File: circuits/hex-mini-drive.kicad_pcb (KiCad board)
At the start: 2 copper layers, 19 parts

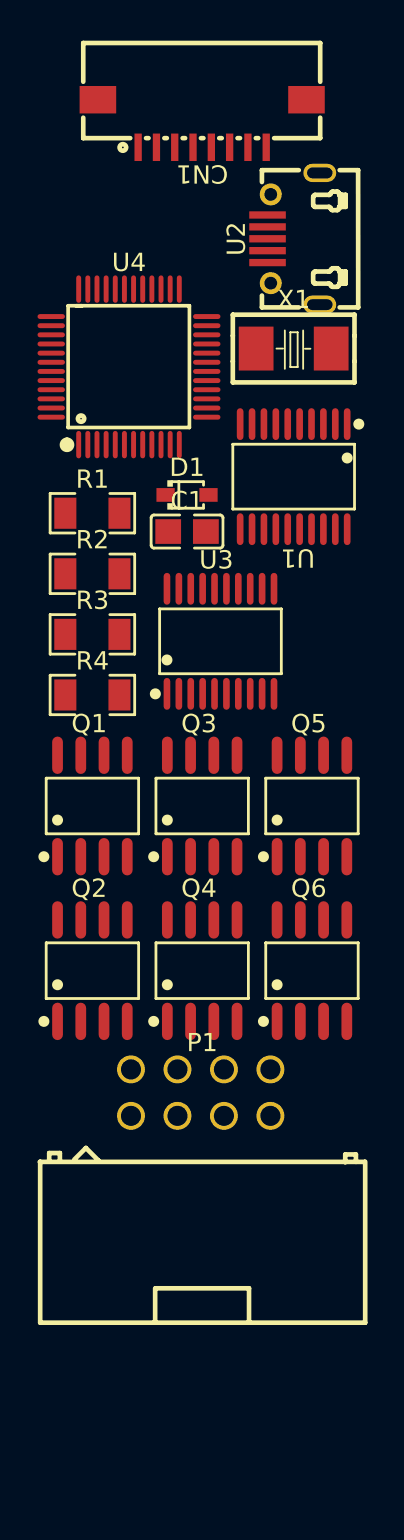
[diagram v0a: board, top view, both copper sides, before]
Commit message: Tentatively complete the PCB layout.
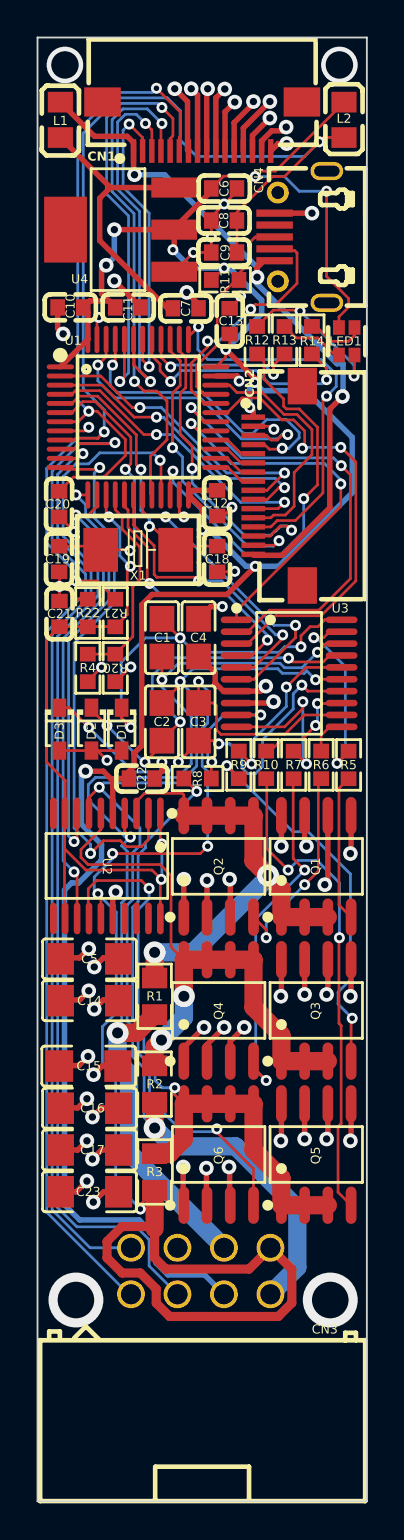
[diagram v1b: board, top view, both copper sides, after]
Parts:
- added C10: 100nF, components_footprints:C0603, F.Cu at (51.8, 64.8)
- added C11: 100nF, components_footprints:C0603, F.Cu at (55.0, 64.8)
- added C12: 100nF, components_footprints:C0603, F.Cu at (59.8, 75.5)
- added C13: 100nF, components_footprints:C0603, F.Cu at (60.5, 65.5)
- added C14: 10uF, components_footprints:C1206, F.Cu at (52.8, 102.6)
- added C15: 10uF, components_footprints:C1206, F.Cu at (52.8, 106.2)
- added C16: 10uF, components_footprints:C1206, F.Cu at (52.8, 108.5)
- added C17: 10uF, components_footprints:C1206, F.Cu at (52.8, 110.8)
- added C18: 30pF, components_footprints:C0603, F.Cu at (59.8, 78.5)
- added C19: 30pF, components_footprints:C0603, F.Cu at (51.2, 78.5)
- added C2: 10nF, components_footprints:C0805, F.Cu at (56.8, 87.4)
- added C20: 100nF, components_footprints:C0603, F.Cu at (51.2, 75.5)
- added C21: 100nF, components_footprints:C0603, F.Cu at (51.2, 81.5)
- added C22: 100nF, components_footprints:C0603, F.Cu at (55.7, 90.5)
- added C23: 10uF, components_footprints:C1206, F.Cu at (52.8, 113.1)
- added C3: 10nF, components_footprints:C0805, F.Cu at (58.8, 87.4)
- added C4: 0.1uF, components_footprints:C0805, F.Cu at (58.8, 82.8)
- added C5: 10uF, components_footprints:C1206, F.Cu at (52.8, 100.4)
- added C6: 1uF, components_footprints:C0603, F.Cu at (60.2, 58.2)
- added C7: 1uF, components_footprints:C0603, F.Cu at (58.1, 64.8)
- added C8: 100nF, components_footprints:C0603, F.Cu at (60.2, 60.0)
- added C9: 1uF, components_footprints:C0603, F.Cu at (60.2, 61.8)
- added CN2: ~, components_footprints:FPC-SMD_P0.50-16P_FGS-XJ-H2.0, F.Cu at (63.1, 74.5)
- added D2: ~, components_footprints:IN4148WS T4 SOD-323_L1.8-W1.3-LS2.5-RD, F.Cu at (53.0, 87.8)
- added D3: ~, components_footprints:IN4148WS T4 SOD-323_L1.8-W1.3-LS2.5-RD, F.Cu at (51.2, 87.8)
- added L1: 300mΩ, components_footprints:L0805, F.Cu at (51.2, 54.5)
- added L2: 10uH, components_footprints:L0805, F.Cu at (66.8, 54.5)
- added LED1: ~, components_footprints:LED-ARRAY-SMD_4P-L1.6-W1.5-BR_XL-1615RGBC-RF, F.Cu at (66.9, 66.6)
- added R10: 10Ω, components_footprints:R0603, F.Cu at (62.5, 89.8)
- added R11: 1.5kΩ, components_footprints:R0603, F.Cu at (60.3, 63.2)
- added R12: 1.5kΩ, components_footprints:R0603, F.Cu at (62.0, 66.5)
- added R13: 1.5kΩ, components_footprints:R0603, F.Cu at (63.5, 66.5)
- added R14: 1.5kΩ, components_footprints:R0603, F.Cu at (65.0, 66.5)
- added R20: 10kΩ, components_footprints:R0603, F.Cu at (54.2, 84.5)
- added R21: 47kΩ, components_footprints:R0603, F.Cu at (54.2, 81.5)
- added R22: 47kΩ, components_footprints:R0603, F.Cu at (52.8, 81.5)
- added R5: 10Ω, components_footprints:R0603, F.Cu at (67.0, 89.8)
- added R6: 10Ω, components_footprints:R0603, F.Cu at (65.5, 89.8)
- added R7: 10Ω, components_footprints:R0603, F.Cu at (64.0, 89.8)
- added R8: 10Ω, components_footprints:R0603, F.Cu at (58.7, 90.5)
- added R9: 10Ω, components_footprints:R0603, F.Cu at (61.0, 89.8)
- added U4: ~, components_footprints:AMS1117-3.3 SOT-223-3_L6.5-W3.4-P2.30-LS7.0-BR, F.Cu at (54.5, 60.5)
- C1: value ~ -> 10nF
- CN1: footprint components_footprints:FPC-SMD_KH-FG1.0-H2.0-8PIN -> components_footprints:FPC-SMD_P0.50-16P_FGS-XJ-H2.0
- R1, R2, R3: value ~ -> 500mW 10mΩ; footprint components_footprints:R1206 -> components_footprints:R0805
- R4: value ~ -> 100kΩ; footprint components_footprints:R1206 -> components_footprints:R0603
- moved R3 29.6 mm to (56.4, 112.0), turned to -90 degrees
- moved R2 28.1 mm to (56.4, 107.2), turned to -90 degrees
- moved R1 26.6 mm to (56.4, 102.4), turned to -90 degrees
- moved Q5 19.0 mm to (65.2, 111.0)
- moved X1 13.9 mm to (55.5, 78.0), turned to 180 degrees
- moved U2 13.8 mm to (53.8, 95.3), turned to 180 degrees
- moved D1 13.3 mm to (54.6, 87.8), turned to -90 degrees
- moved Q3 12.8 mm to (65.2, 103.2)
- moved Q1 12.7 mm to (65.2, 95.3)
- moved Q6 11.3 mm to (59.9, 111.0)
- moved U3 10.8 mm to (63.8, 84.8), turned to -90 degrees
- moved CN3 9.75 mm to (58.9, 117.4)
- moved Q2 8.95 mm to (59.9, 95.3)
- moved C1 5.96 mm to (56.8, 82.8), turned to 90 degrees
- moved U1 2.80 mm to (55.5, 70.8), turned to -90 degrees
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- renumbered P1 to CN3, U2 to CN4, U4 to U1, U3 to U2, U1 to U3
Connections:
- C1 pad 1: unconnected-(C1-Pad1) -> OUT1
- C1 pad 2: unconnected-(C1-Pad2) -> /Boost Gate 1
- CN1 pad 1: unconnected-(CN1-Pad1) -> +5V
- CN1 pad 10: unconnected-(CN1-Pad10) -> GND
- CN1 pad 2: unconnected-(CN1-Pad2) -> USART1_TX
- CN1 pad 3: unconnected-(CN1-Pad3) -> USART1_RX
- CN1 pad 4: unconnected-(CN1-Pad4) -> GPIO_Input_CS
- CN1 pad 5: unconnected-(CN1-Pad5) -> BOOT0
- CN1 pad 6: unconnected-(CN1-Pad6) -> NRST
- CN1 pad 7: unconnected-(CN1-Pad7) -> GND
- CN1 pad 8: unconnected-(CN1-Pad8) -> GND
- CN1 pad 9: unconnected-(CN1-Pad9) -> GND
- CN3 pad 1: unconnected-(P1-Pad1) -> TIM2_CH1/H1
- CN3 pad 2: unconnected-(P1-Pad2) -> TIM2_CH2/H2
- CN3 pad 3: unconnected-(P1-Pad3) -> TIM2_CH3/H3
- CN3 pad 4: unconnected-(P1-Pad4) -> GND
- CN3 pad 5: unconnected-(P1-Pad5) -> +3V3
- CN3 pad 6: unconnected-(P1-Pad6) -> OUT1
- CN3 pad 7: unconnected-(P1-Pad7) -> OUT2
- CN3 pad 8: unconnected-(P1-Pad8) -> OUT3
- CN4 pad 1: unconnected-(U2-VCC-Pad1) -> +5V
- CN4 pad 2: unconnected-(U2-D--Pad2) -> USB_D-
- CN4 pad 3: unconnected-(U2-D+-Pad3) -> USB_D+
- CN4 pad 5: unconnected-(U2-GND-Pad5) -> GND
- D1 pad 1: unconnected-(D1-K-Pad1) -> /Boost Gate 1
- D1 pad 2: unconnected-(D1-A-Pad2) -> +VDC
- Q1 pad 1: unconnected-(Q1-S-Pad1) -> SHUNT1
- Q1 pad 2: unconnected-(Q1-S-Pad2) -> SHUNT1
- Q1 pad 3: unconnected-(Q1-S-Pad3) -> SHUNT1
- Q1 pad 4: unconnected-(Q1-G-Pad4) -> GATE1H
- Q1 pad 5: unconnected-(Q1-D-Pad5) -> +VDC
- Q1 pad 6: unconnected-(Q1-D-Pad6) -> +VDC
- Q1 pad 7: unconnected-(Q1-D-Pad7) -> +VDC
- Q1 pad 8: unconnected-(Q1-D-Pad8) -> +VDC
- Q2 pad 1: unconnected-(Q2-S-Pad1) -> GND
- Q2 pad 2: unconnected-(Q2-S-Pad2) -> GND
- Q2 pad 3: unconnected-(Q2-S-Pad3) -> GND
- Q2 pad 4: unconnected-(Q2-G-Pad4) -> GATE1L
- Q2 pad 5: unconnected-(Q2-D-Pad5) -> SHUNT1
- Q2 pad 6: unconnected-(Q2-D-Pad6) -> SHUNT1
- Q2 pad 7: unconnected-(Q2-D-Pad7) -> SHUNT1
- Q2 pad 8: unconnected-(Q2-D-Pad8) -> SHUNT1
- Q3 pad 1: unconnected-(Q3-S-Pad1) -> SHUNT2
- Q3 pad 2: unconnected-(Q3-S-Pad2) -> SHUNT2
- Q3 pad 3: unconnected-(Q3-S-Pad3) -> SHUNT2
- Q3 pad 4: unconnected-(Q3-G-Pad4) -> GATE2H
- Q3 pad 5: unconnected-(Q3-D-Pad5) -> +VDC
- Q3 pad 6: unconnected-(Q3-D-Pad6) -> +VDC
- Q3 pad 7: unconnected-(Q3-D-Pad7) -> +VDC
- Q3 pad 8: unconnected-(Q3-D-Pad8) -> +VDC
- Q4 pad 1: unconnected-(Q4-S-Pad1) -> GND
- Q4 pad 2: unconnected-(Q4-S-Pad2) -> GND
- Q4 pad 3: unconnected-(Q4-S-Pad3) -> GND
- Q4 pad 4: unconnected-(Q4-G-Pad4) -> GATE2L
- Q4 pad 5: unconnected-(Q4-D-Pad5) -> SHUNT2
- Q4 pad 6: unconnected-(Q4-D-Pad6) -> SHUNT2
- Q4 pad 7: unconnected-(Q4-D-Pad7) -> SHUNT2
- Q4 pad 8: unconnected-(Q4-D-Pad8) -> SHUNT2
- Q5 pad 1: unconnected-(Q5-S-Pad1) -> SHUNT3
- Q5 pad 2: unconnected-(Q5-S-Pad2) -> SHUNT3
- Q5 pad 3: unconnected-(Q5-S-Pad3) -> SHUNT3
- Q5 pad 4: unconnected-(Q5-G-Pad4) -> GATE3H
- Q5 pad 5: unconnected-(Q5-D-Pad5) -> +VDC
- Q5 pad 6: unconnected-(Q5-D-Pad6) -> +VDC
- Q5 pad 7: unconnected-(Q5-D-Pad7) -> +VDC
- Q5 pad 8: unconnected-(Q5-D-Pad8) -> +VDC
- Q6 pad 1: unconnected-(Q6-S-Pad1) -> GND
- Q6 pad 2: unconnected-(Q6-S-Pad2) -> GND
- Q6 pad 3: unconnected-(Q6-S-Pad3) -> GND
- Q6 pad 4: unconnected-(Q6-G-Pad4) -> GATE3L
- Q6 pad 5: unconnected-(Q6-D-Pad5) -> SHUNT3
- Q6 pad 6: unconnected-(Q6-D-Pad6) -> SHUNT3
- Q6 pad 7: unconnected-(Q6-D-Pad7) -> SHUNT3
- Q6 pad 8: unconnected-(Q6-D-Pad8) -> SHUNT3
- R1 pad 1: unconnected-(R1-Pad1) -> SHUNT1
- R1 pad 2: unconnected-(R1-Pad2) -> OUT1
- R2 pad 1: unconnected-(R2-Pad1) -> SHUNT2
- R2 pad 2: unconnected-(R2-Pad2) -> OUT2
- R3 pad 1: unconnected-(R3-Pad1) -> SHUNT3
- R3 pad 2: unconnected-(R3-Pad2) -> OUT3
- R4 pad 1: unconnected-(R4-Pad1) -> ADC1_IN6
- R4 pad 2: unconnected-(R4-Pad2) -> +VDC
- U1 pad 1: unconnected-(U4-VBAT-Pad1) -> +3V3
- U1 pad 10: unconnected-(U4-PA0-WKUP-Pad10) -> TIM2_CH1/H1
- U1 pad 11: unconnected-(U4-PA1-Pad11) -> TIM2_CH2/H2
- U1 pad 12: unconnected-(U4-PA2-Pad12) -> ADC1_IN2
- U1 pad 13: unconnected-(U4-PA3-Pad13) -> ADC1_IN3
- U1 pad 14: unconnected-(U4-PA4-Pad14) -> ADC1_IN4
- U1 pad 15: unconnected-(U4-PA5-Pad15) -> ADC1_IN5/REF
- U1 pad 16: unconnected-(U4-PA6-Pad16) -> ADC1_IN6
- U1 pad 17: unconnected-(U4-PA7-Pad17) -> TIM1_CH1N
- U1 pad 18: unconnected-(U4-PB0-Pad18) -> TIM1_CH2N
- U1 pad 19: unconnected-(U4-PB1-Pad19) -> TIM1_CH3N
- U1 pad 2: unconnected-(U4-PC13-TAMPER-RTC-Pad2) -> GPIO_Input_A
- U1 pad 20: unconnected-(U4-PB2-Pad20) -> GPIO_Input_CS
- U1 pad 21: unconnected-(U4-PB10-Pad21) -> TIM2_CH3/H3
- U1 pad 22: unconnected-(U4-PB11-Pad22) -> TIM2_CH4
- U1 pad 23: unconnected-(U4-VSS_1-Pad23) -> GND
- U1 pad 24: unconnected-(U4-VDD_1-Pad24) -> +3V3
- U1 pad 25: unconnected-(U4-PB12-Pad25) -> SPI2_NSS
- U1 pad 26: unconnected-(U4-PB13-Pad26) -> SPI2_SCK
- U1 pad 27: unconnected-(U4-PB14-Pad27) -> SPI2MISO
- U1 pad 28: unconnected-(U4-PB15-Pad28) -> SPI2_MOSI
- U1 pad 29: unconnected-(U4-PA8-Pad29) -> TIM1_CH1
- U1 pad 3: unconnected-(U4-PC14-OSC32_IN-Pad3) -> GPIO_Input_B
- U1 pad 30: unconnected-(U4-PA9-Pad30) -> TIM1_CH2
- U1 pad 31: unconnected-(U4-PA10-Pad31) -> TIM1_CH3
- U1 pad 32: unconnected-(U4-PA11-Pad32) -> USB_D-
- U1 pad 33: unconnected-(U4-PA12-Pad33) -> USB_D+
- U1 pad 34: unconnected-(U4-PA13-Pad34) -> SYS_JTMS-SWDIO
- U1 pad 35: unconnected-(U4-VSS_2-Pad35) -> GND
- U1 pad 36: unconnected-(U4-VDD_2-Pad36) -> +3V3
- U1 pad 37: unconnected-(U4-PA14-Pad37) -> SYS_JTCK-SWCLK
- U1 pad 38: unconnected-(U4-PA15-Pad38) -> SYS_JTDI
- U1 pad 39: unconnected-(U4-PB3-Pad39) -> SYS_JTDO-TRACESWO
- U1 pad 4: unconnected-(U4-PC15-OSC32_OUT-Pad4) -> GPIO_Input_C
- U1 pad 40: unconnected-(U4-PB4-Pad40) -> TIM3_CH1
- U1 pad 41: unconnected-(U4-PB5-Pad41) -> TIM3_CH2
- U1 pad 42: unconnected-(U4-PB6-Pad42) -> USART1_TX
- U1 pad 43: unconnected-(U4-PB7-Pad43) -> USART1_RX
- U1 pad 44: unconnected-(U4-BOOT0-Pad44) -> BOOT0
- U1 pad 45: unconnected-(U4-PB8-Pad45) -> I2C1_SCL
- U1 pad 46: unconnected-(U4-PB9-Pad46) -> I2C1_SDA
- U1 pad 47: unconnected-(U4-VSS_3-Pad47) -> GND
- U1 pad 48: unconnected-(U4-VDD_3-Pad48) -> +3V3
- U1 pad 5: unconnected-(U4-PD0-OSC_IN-Pad5) -> /RCC_OSC_IN
- U1 pad 6: unconnected-(U4-PD1-OSC_OUT-Pad6) -> /RCC_OSC_OUT
- U1 pad 7: unconnected-(U4-NRST-Pad7) -> NRST
- U1 pad 8: unconnected-(U4-VSSA-Pad8) -> GND
- U1 pad 9: unconnected-(U4-VDDA-Pad9) -> +3V3A
- U2 pad 1: unconnected-(U3-REF1-Pad1) -> ADC1_IN5/REF
- U2 pad 12: unconnected-(U3-REF3-Pad12) -> ADC1_IN5/REF
- U2 pad 13: unconnected-(U3-OUT3-Pad13) -> ADC1_IN4
- U2 pad 14: unconnected-(U3-IN±3-Pad14) -> SHUNT3
- U2 pad 15: unconnected-(U3-IN+3-Pad15) -> OUT3
- U2 pad 16: unconnected-(U3-GND-Pad16) -> GND
- U2 pad 2: unconnected-(U3-OUT1-Pad2) -> ADC1_IN2
- U2 pad 20: unconnected-(U3-REF4-Pad20) -> ADC1_IN5/REF
- U2 pad 3: unconnected-(U3-IN±1-Pad3) -> SHUNT1
- U2 pad 4: unconnected-(U3-IN+1-Pad4) -> OUT1
- U2 pad 5: unconnected-(U3-VS-Pad5) -> +3V3
- U2 pad 6: unconnected-(U3-IN+2-Pad6) -> SHUNT2
- U2 pad 7: unconnected-(U3-IN±2-Pad7) -> OUT2
- U2 pad 8: unconnected-(U3-OUT2-Pad8) -> ADC1_IN3
- U2 pad 9: unconnected-(U3-REF2-Pad9) -> ADC1_IN5/REF
- U3 pad 1: unconnected-(U1-HIN1-Pad1) -> TIM1_CH1
- U3 pad 10: unconnected-(U1-LO2-Pad10) -> /LO2
- U3 pad 11: unconnected-(U1-LO1-Pad11) -> /LO1
- U3 pad 12: unconnected-(U1-VS3-Pad12) -> OUT3
- U3 pad 13: unconnected-(U1-HO3-Pad13) -> /HO3
- U3 pad 14: unconnected-(U1-VB3-Pad14) -> /Boost Gate 3
- U3 pad 15: unconnected-(U1-VS2-Pad15) -> OUT2
- U3 pad 16: unconnected-(U1-HO2-Pad16) -> /HO2
- U3 pad 17: unconnected-(U1-VB2-Pad17) -> /Boost Gate 2
- U3 pad 18: unconnected-(U1-VS1-Pad18) -> OUT1
- U3 pad 19: unconnected-(U1-HO1-Pad19) -> /HO1
- U3 pad 2: unconnected-(U1-HIN2-Pad2) -> TIM1_CH2
- U3 pad 20: unconnected-(U1-VB1-Pad20) -> /Boost Gate 1
- U3 pad 3: unconnected-(U1-HIN3-Pad3) -> TIM1_CH3
- U3 pad 4: unconnected-(U1-LIN1-Pad4) -> TIM1_CH1N
- U3 pad 5: unconnected-(U1-LIN2-Pad5) -> TIM1_CH2N
- U3 pad 6: unconnected-(U1-LIN3-Pad6) -> TIM1_CH3N
- U3 pad 7: unconnected-(U1-VCC-Pad7) -> +VDC
- U3 pad 8: unconnected-(U1-COM-Pad8) -> GND
- U3 pad 9: unconnected-(U1-LO3-Pad9) -> /LO3
- X1 pad 1: unconnected-(X1-OSC1-Pad1) -> /RCC_OSC_IN
- X1 pad 2: unconnected-(X1-OSC2-Pad2) -> /RCC_OSC_OUT
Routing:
- net +3V3: track 0.00 -> 139.8 mm, vias 0 -> 12
- net GND: track 0.00 -> 81.5 mm, vias 0 -> 43
- net OUT3: track 0.00 -> 80.3 mm, vias 0 -> 5
- net OUT2: track 0.00 -> 60.5 mm, vias 0 -> 4
- net TIM2_CH3/H3: track 0.00 -> 58.9 mm, vias 0 -> 1
- net +3V3A: track 0.00 -> 58.8 mm, vias 0 -> 3
- net +VDC: track 0.00 -> 57.1 mm, vias 0 -> 27
- net OUT1: track 0.00 -> 56.7 mm, vias 0 -> 4
- net TIM2_CH1/H1: track 0.00 -> 55.8 mm, vias 0 -> 1
- net TIM2_CH2/H2: track 0.00 -> 50.2 mm, vias 0 -> 1
- net ADC1_IN5/REF: track 0.00 -> 41.5 mm, vias 0 -> 4
- net +5V: track 0.00 -> 38.1 mm, vias 0 -> 3
- net SHUNT3: track 0.00 -> 35.2 mm, vias 0 -> 2
- net NRST: track 0.00 -> 34.6 mm, vias 0 -> 2
- net SHUNT2: track 0.00 -> 32.1 mm, vias 0 -> 2
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- added copper zone on In2.Cu, net +VDC
- added copper zone on In1.Cu, net GND
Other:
- board outline added: 18 x 80 mm
- copper layers 2 -> 4
